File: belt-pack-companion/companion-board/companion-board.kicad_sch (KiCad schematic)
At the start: 4 parts, among them J1 Conn_01x18_Socket, J2 Conn_01x18_Socket, J3 AudioJack4_Ground, U1 TLV320AIC3204

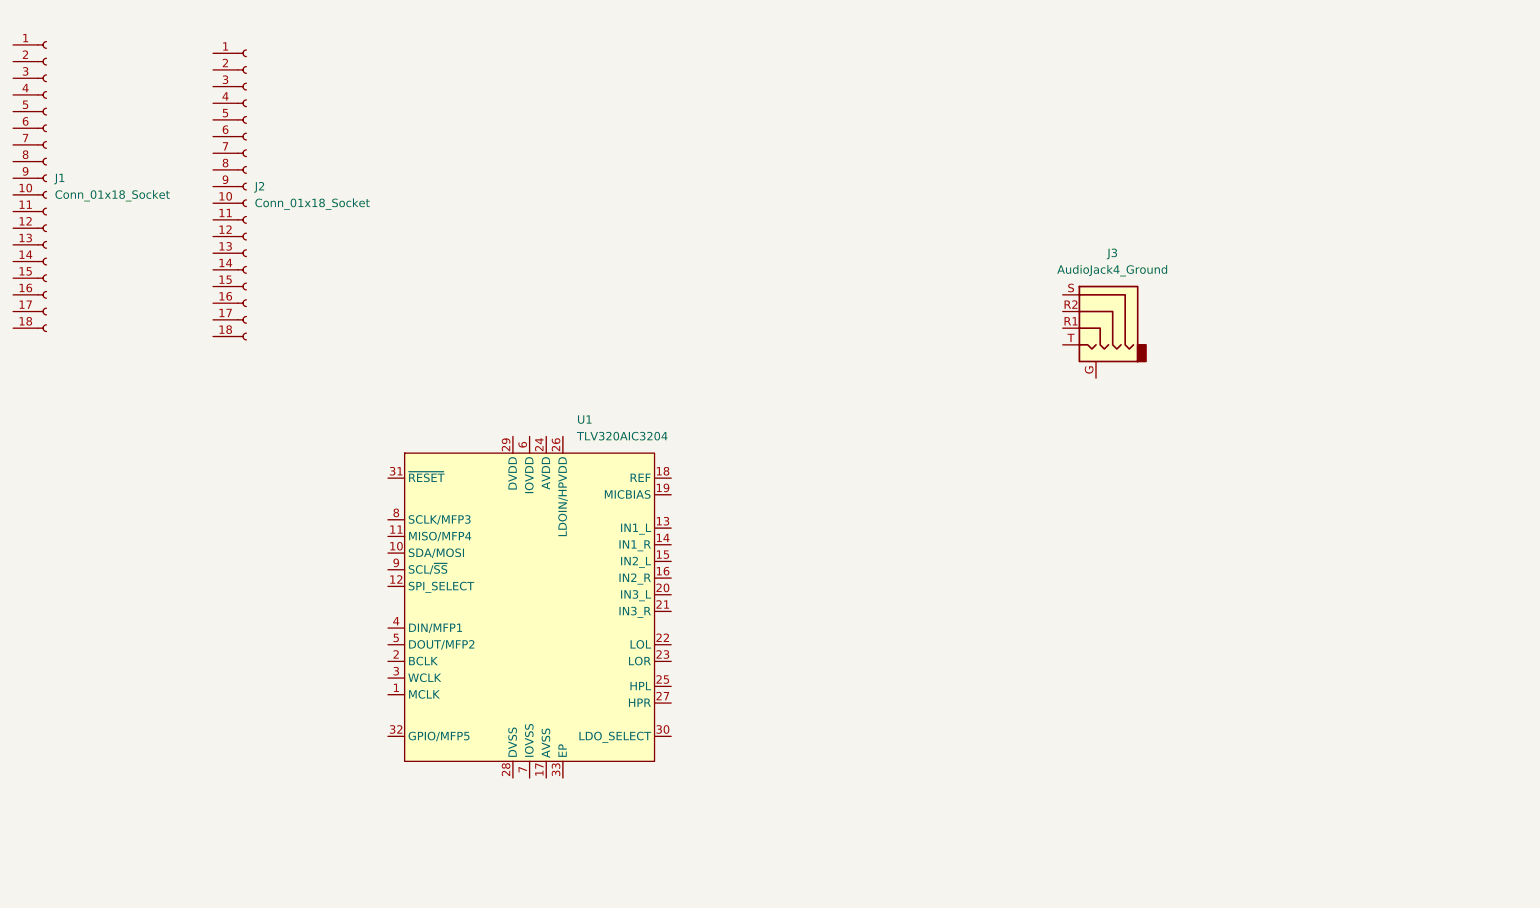
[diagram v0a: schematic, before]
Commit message: companion board update
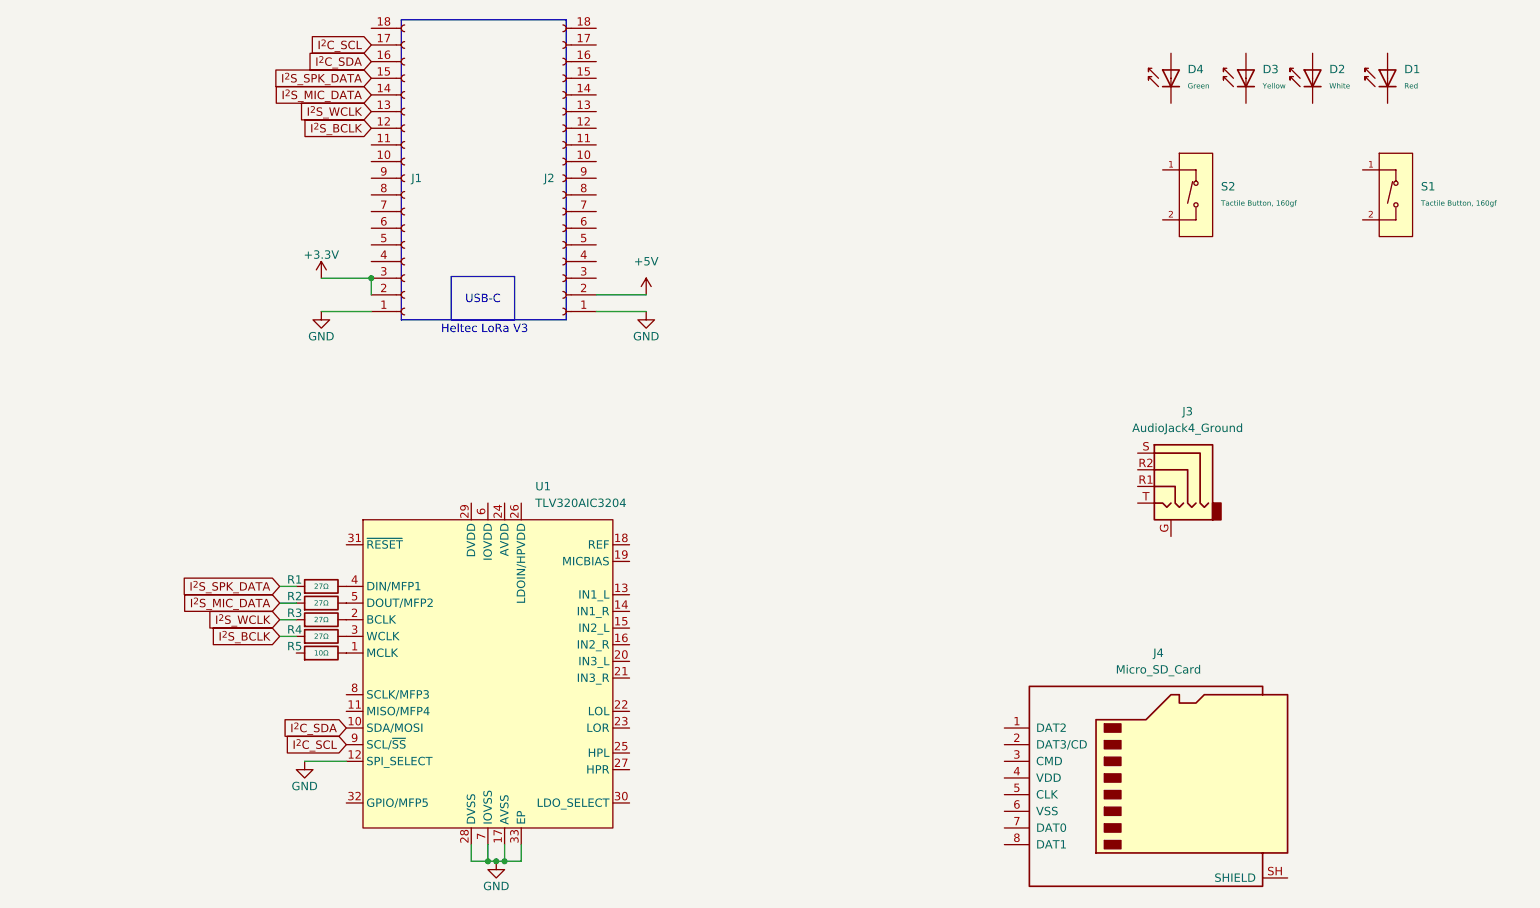
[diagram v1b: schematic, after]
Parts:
- added D1: Red, PCM_JLCPCB:D_0603, symbol PCM_JLCPCB-Diodes:LED,0603,Red
- added D2: White, PCM_JLCPCB:D_0603, symbol PCM_JLCPCB-Diodes:LED,0603,White
- added D3: Yellow, PCM_JLCPCB:D_0603, symbol PCM_JLCPCB-Diodes:LED,0603,Yellow
- added D4: Green, PCM_JLCPCB:D_0805, symbol PCM_JLCPCB-Diodes:LED,0805,Green
- added J4: Micro_SD_Card, symbol Connector:Micro_SD_Card
- added R1, R2, R3, R4: 27Ω, PCM_JLCPCB:R_0603, symbol PCM_JLCPCB-Resistors:0603,27Ω
- added R5: 10Ω, PCM_JLCPCB:R_0603, symbol PCM_JLCPCB-Resistors:0603,10Ω
- added S1, S2: Tactile Button, 160gf, PCM_JLCPCB:SW_TS-1088-AR02016, symbol PCM_JLCPCB-Connectors_Buttons:Tactile Button, 160gf, 12V, 50mA, 4.0mm
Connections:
- net GND: now reaches J2.1 (Pin_1)
- net GND: now also J1.1 (Pin_1), U1.12 (SPI_SELECT), U1.17 (AVSS), U1.28 (DVSS), U1.33 (EP), U1.7 (IOVSS)
- net +5V: now reaches J2.2 (Pin_2)
- net at U1.1 (MCLK): now also R5.2
- net I^{2}C_SDA: now reaches U1.10 (SDA/MOSI)
- net I^{2}C_SDA: now also J1.16 (Pin_16)
- net at U1.2 (BCLK): now also R3.2
- net at U1.3 (WCLK): now also R4.2
- net at U1.4 (DIN/MFP1): now also R1.2
- net at U1.5 (DOUT/MFP2): now also R2.2
- net I^{2}C_SCL: now reaches U1.9 (SCL/~{SS})
- net I^{2}C_SCL: now also J1.17 (Pin_17)
- net I^{2}S_BCLK: now reaches J1.12 (Pin_12)
- net I^{2}S_BCLK: now also R4.1
- net I^{2}S_WCLK: now reaches J1.13 (Pin_13)
- net I^{2}S_WCLK: now also R3.1
- net I^{2}S_MIC_DATA: now reaches J1.14 (Pin_14)
- net I^{2}S_MIC_DATA: now also R2.1
- net I^{2}S_SPK_DATA: now reaches J1.15 (Pin_15)
- net I^{2}S_SPK_DATA: now also R1.1
- net +3.3V: now reaches J1.2 (Pin_2)
- net +3.3V: now also J1.3 (Pin_3)
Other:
- note added: "Heltec LoRa V3"
- note added: "USB-C"
- moved on the sheet: J1, J2, J3, U1
